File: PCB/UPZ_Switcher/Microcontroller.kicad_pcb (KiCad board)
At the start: 2 copper layers, 17 parts, among them IC1 MAX232ECPE+, J1 5747844-6, SW1 SW_DIP_x04, SW2 SW_DIP_x04

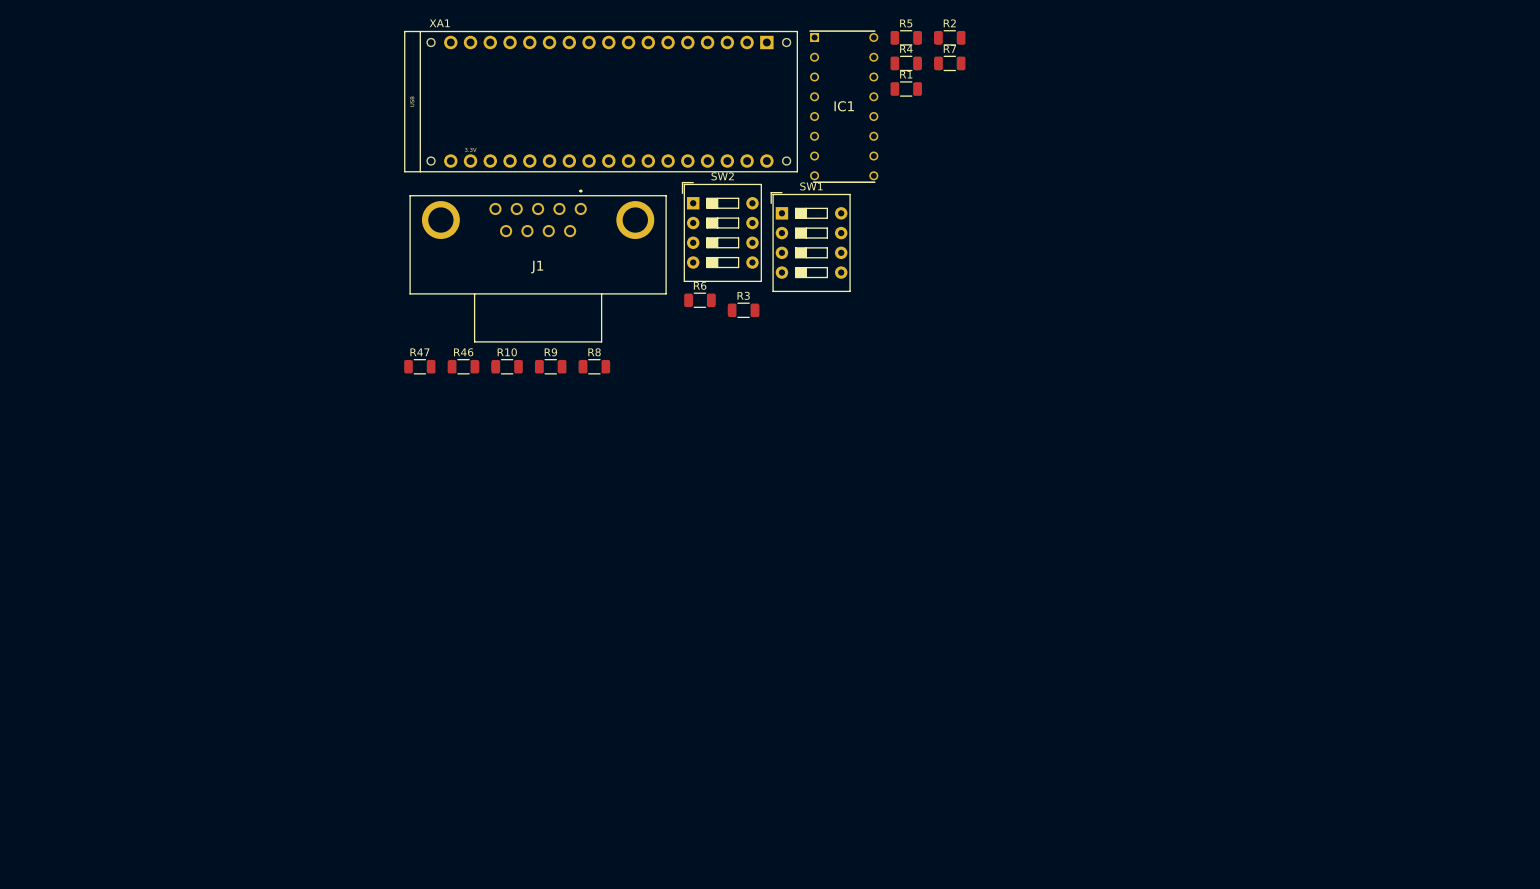
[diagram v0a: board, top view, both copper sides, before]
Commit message: updated phantom design + MCU board
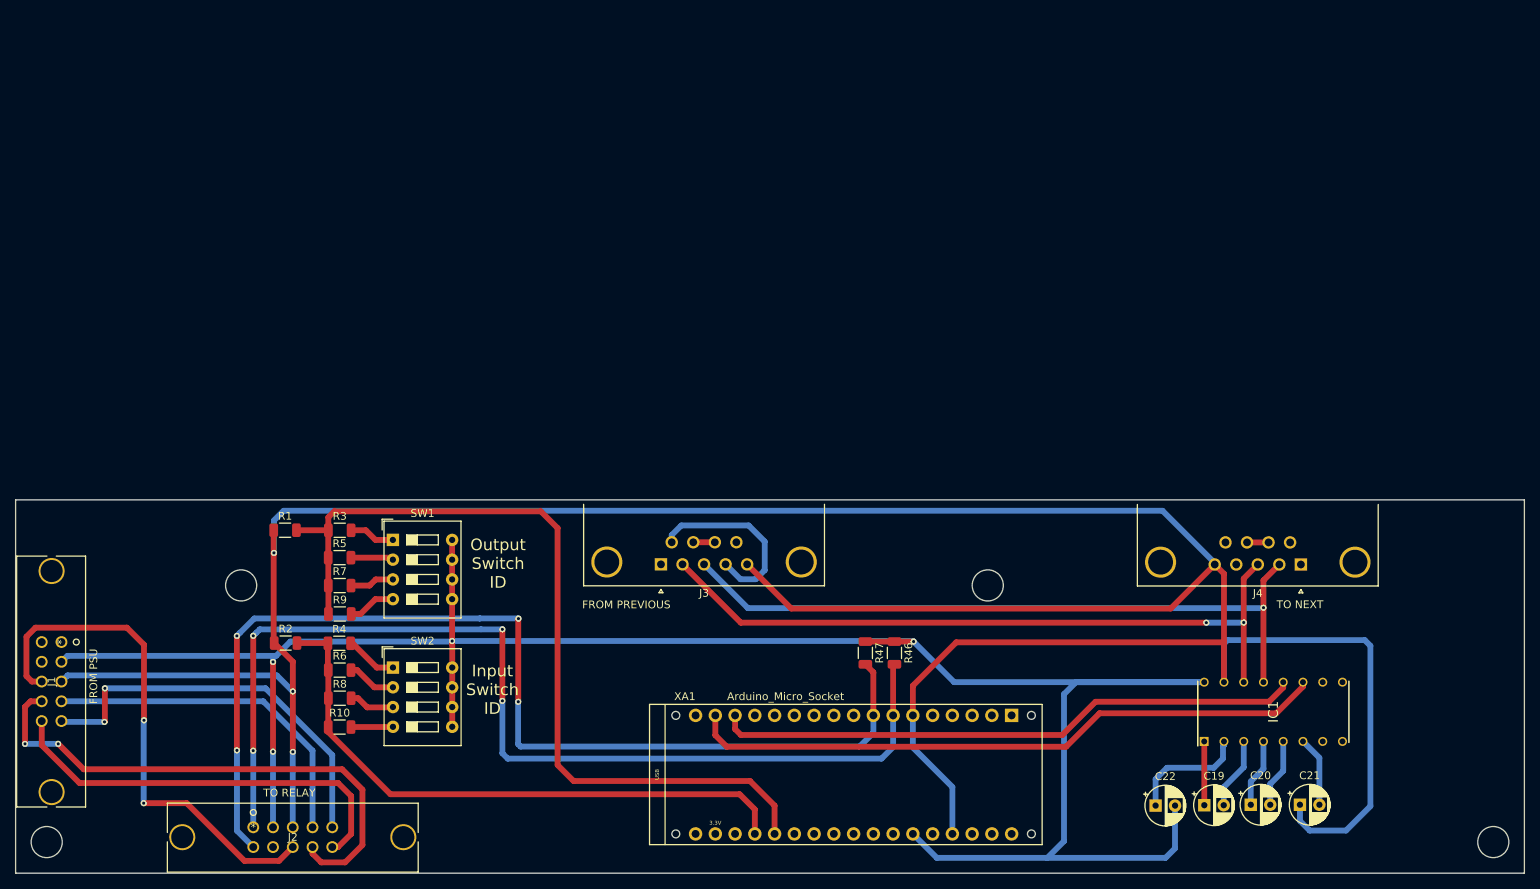
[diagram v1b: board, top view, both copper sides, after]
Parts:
- added C19: 1uF, Capacitor_THT:CP_Radial_D5.0mm_P2.50mm, F.Cu at (188.5, 143.6)
- added C20: 1uF, Capacitor_THT:CP_Radial_D5.0mm_P2.50mm, F.Cu at (194.5, 143.5)
- added C21: 1uF, Capacitor_THT:CP_Radial_D5.0mm_P2.50mm, F.Cu at (200.8, 143.5)
- added C22: 1uF, Capacitor_THT:CP_Radial_D5.0mm_P2.50mm, F.Cu at (182.3, 143.6)
- added J2: TO RELAY, BVKSound:71918-110LF, F.Cu at (66.2, 146.4)
- added J3: FROM PREVIOUS, Connector_Dsub:DSUB-9_Female_Horizontal_P2.77x2.84mm_EdgePinOffset4.94mm_Housed_MountingHolesOffset7.48mm, F.Cu at (118.7, 112.6)
- added J4: TO NEXT, Connector_Dsub:DSUB-9_Male_Horizontal_P2.77x2.84mm_EdgePinOffset4.94mm_Housed_MountingHolesOffset7.48mm, F.Cu at (200.9, 112.6)
- J1: value 5747844-6 -> FROM PSU; footprint BVKSound:57478446 -> BVKSound:71918-110LF
- moved R2 115.5 mm to (70.4, 122.7)
- moved R4 104.3 mm to (77.3, 122.7)
- moved R7 103.3 mm to (77.4, 115.3)
- moved R5 98.9 mm to (77.3, 111.7)
- moved R1 98.0 mm to (70.3, 108.2)
- moved IC1 95.4 mm to (197.4, 131.5), turned to 90 degrees
- moved XA1 92.1 mm to (119.2, 148.6)
- moved J1 78.1 mm to (41.6, 122.6), turned to 270 degrees
- moved SW2 71.1 mm to (84.2, 125.8)
- moved R47 68.1 mm to (144.9, 124.0), turned to 270 degrees
- moved R46 66.5 mm to (148.7, 124.0), turned to 270 degrees
- moved R6 66.4 mm to (77.4, 126.2)
- moved SW1 65.3 mm to (84.2, 109.4)
- moved R3 59.1 mm to (77.4, 108.2)
- moved R8 53.7 mm to (77.4, 129.8)
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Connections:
- J1 pad 2: Net-(IC1-Pad14) -> Net-(J1-Pad2)
- J1 pad 3: Net-(IC1-Pad13) -> /5V
- J1 pad 6: Net-(J1-Pad4) -> Net-(J1-Pad6)
- J1 pad 8: Net-(J1-Pad7) -> Net-(J1-Pad8)
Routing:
- net GND: track 0.00 -> 400.7 mm, vias 0 -> 3
- net /5V: track 0.00 -> 284.6 mm, vias 0 -> 4
- net /I2C_SCK: track 0.00 -> 137.1 mm, vias 0 -> 4
- net /I2C_SDA: track 0.00 -> 134.8 mm, vias 0 -> 4
- net Net-(R1-Pad2): track 0.00 -> 111.4 mm
- net Net-(IC1-Pad14): track 0.00 -> 91.2 mm, vias 0 -> 2
- net Net-(IC1-Pad13): track 0.00 -> 90.3 mm, vias 0 -> 1
- net Net-(IC1-Pad11): track 0.00 -> 82.5 mm
- net Net-(R10-Pad1): track 0.00 -> 77.5 mm
- net Net-(IC1-Pad12): track 0.00 -> 75.8 mm
- net Net-(J1-Pad8): track 0.00 -> 68.8 mm, vias 0 -> 2
- net Net-(J1-Pad6): track 0.00 -> 67.2 mm, vias 0 -> 2
- net Net-(J1-Pad10): track 0.00 -> 53.6 mm
- net Net-(J1-Pad9): track 0.00 -> 52.0 mm, vias 0 -> 2
- net Net-(J1-Pad7): track 0.00 -> 44.8 mm
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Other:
- board outline added: 194 x 48 mm
- board text added: "Input Switch ID"
- board text added: "Output Switch ID"
